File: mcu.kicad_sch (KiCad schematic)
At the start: 42 parts, among them SW1 TS-1088-AR02016, SW2 TS-1088-AR02016, SW3 TS-1088-AR02016, SW4 TS-1088-AR02016, U1 STM32H723VGTx, U14 AS5047P-ATST, U15 TCAN1044VDRQ1, U9 LSM6DSVTR, X1 X322512MSB4SI

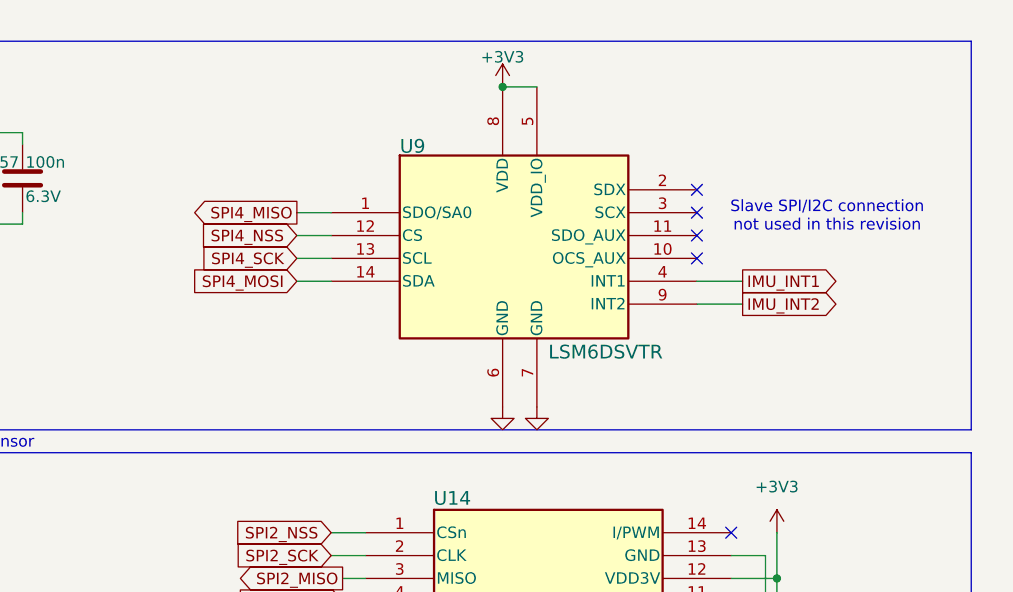
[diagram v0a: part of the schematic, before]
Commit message: wip gate driver change
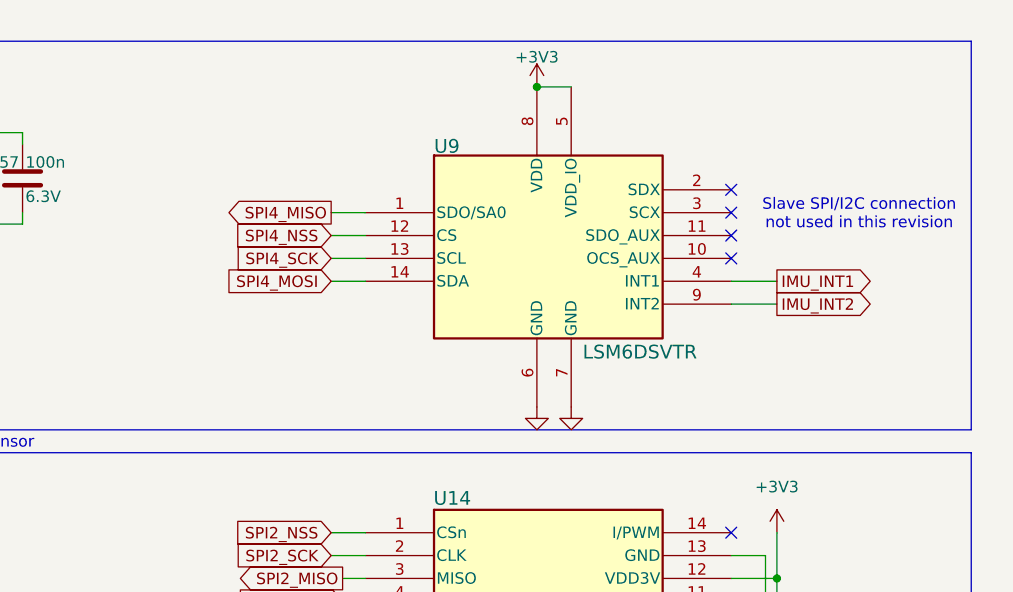
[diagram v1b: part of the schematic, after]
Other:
- moved on the sheet: U9
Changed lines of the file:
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@@
 	(text "Slave SPI/I2C connection\nnot used in this revision"
 		(exclude_from_sim no)
-		(at 265.938 34.798 0)
+		(at 269.494 34.544 0)
 		(effects
 			(font
@@
 	)
 	(junction
-		(at 229.87 20.32)
+		(at 233.68 20.32)
 		(diameter 0)
 		(color 0 0 0 0)
@@
 	)
 	(no_connect
-		(at 251.46 39.37)
+		(at 255.27 39.37)
 	)
 	(no_connect
-		(at 251.46 36.83)
+		(at 255.27 36.83)
 	)
 	(no_connect
@@
 	)
 	(no_connect
-		(at 251.46 31.75)
+		(at 255.27 31.75)
 	)
 	(no_connect
@@
 	)
 	(no_connect
-		(at 251.46 34.29)
+		(at 255.27 34.29)
 	)
 	(no_connect
@@
 	(wire
 		(pts
-			(xy 207.01 39.37) (xy 210.82 39.37)
+			(xy 210.82 39.37) (xy 214.63 39.37)
 		)
 		(stroke
@@
 	(wire
 		(pts
-			(xy 207.01 41.91) (xy 210.82 41.91)
+			(xy 210.82 41.91) (xy 214.63 41.91)
 		)
 		(stroke
@@
 	(wire
 		(pts
-			(xy 229.87 20.32) (xy 233.68 20.32)
+			(xy 233.68 20.32) (xy 237.49 20.32)
 		)
 		(stroke
@@
 	(wire
 		(pts
-			(xy 251.46 44.45) (xy 256.54 44.45)
+			(xy 255.27 44.45) (xy 260.35 44.45)
 		)
 		(stroke
@@
 	(wire
 		(pts
-			(xy 251.46 41.91) (xy 256.54 41.91)
+			(xy 255.27 41.91) (xy 260.35 41.91)
 		)
 		(stroke
@@
 	(wire
 		(pts
-			(xy 207.01 34.29) (xy 210.82 34.29)
+			(xy 210.82 34.29) (xy 214.63 34.29)
 		)
 		(stroke
@@
 	(wire
 		(pts
-			(xy 207.01 36.83) (xy 210.82 36.83)
+			(xy 210.82 36.83) (xy 214.63 36.83)
 		)
 		(stroke
@@
 	(global_label "SPI4_MOSI"
 		(shape input)
-		(at 207.01 41.91 180)
+		(at 210.82 41.91 180)
 		(fields_autoplaced yes)
 		(effects
@@
 		)
 		(property "Intersheetrefs" "${INTERSHEET_REFS}"
-			(at 194.1672 41.91 0)
+			(at 197.9772 41.91 0)
 			(effects
 				(font
@@
 	(global_label "IMU_INT2"
 		(shape output)
-		(at 256.54 44.45 0)
+		(at 260.35 44.45 0)
 		(fields_autoplaced yes)
 		(effects
@@
 		)
 		(property "Intersheetrefs" "${INTERSHEET_REFS}"
-			(at 267.9919 44.45 0)
+			(at 271.8019 44.45 0)
 			(effects
 				(font
@@
 	(global_label "SPI4_SCK"
 		(shape input)
-		(at 207.01 39.37 180)
+		(at 210.82 39.37 180)
 		(fields_autoplaced yes)
 		(effects
@@
 		)
 		(property "Intersheetrefs" "${INTERSHEET_REFS}"
-			(at 195.0139 39.37 0)
+			(at 198.8239 39.37 0)
 			(effects
 				(font
@@
 	(global_label "IMU_INT1"
 		(shape output)
-		(at 256.54 41.91 0)
+		(at 260.35 41.91 0)
 		(fields_autoplaced yes)
 		(effects
@@
 		)
 		(property "Intersheetrefs" "${INTERSHEET_REFS}"
-			(at 267.9919 41.91 0)
+			(at 271.8019 41.91 0)
 			(effects
 				(font
@@
 	(global_label "SPI4_MISO"
 		(shape output)
-		(at 207.01 34.29 180)
+		(at 210.82 34.29 180)
 		(fields_autoplaced yes)
 		(effects
@@
 		)
 		(property "Intersheetrefs" "${INTERSHEET_REFS}"
-			(at 194.1672 34.29 0)
+			(at 197.9772 34.29 0)
 			(effects
 				(font
@@
 	(global_label "SPI4_NSS"
 		(shape input)
-		(at 207.01 36.83 180)
+		(at 210.82 36.83 180)
 		(fields_autoplaced yes)
 		(effects
@@
 		)
 		(property "Intersheetrefs" "${INTERSHEET_REFS}"
-			(at 195.0139 36.83 0)
+			(at 198.8239 36.83 0)
 			(effects
 				(font
@@
 	(symbol
 		(lib_id "power:+3V3")
-		(at 229.87 20.32 0)
+		(at 233.68 20.32 0)
 		(unit 1)
 		(exclude_from_sim no)
@@
 		(dnp no)
 		(property "Reference" "#PWR0134"
-			(at 229.87 24.13 0)
+			(at 233.68 24.13 0)
 			(effects
 				(font
@@
 		)
 		(property "Value" "+3V3"
-			(at 229.87 17.018 0)
+			(at 233.68 17.018 0)
 			(effects
 				(font
@@
 		)
 		(property "Footprint" ""
-			(at 229.87 20.32 0)
+			(at 233.68 20.32 0)
 			(effects
 				(font
@@
 		)
 		(property "Datasheet" ""
-			(at 229.87 20.32 0)
+			(at 233.68 20.32 0)
 			(effects
 				(font
@@
 		)
 		(property "Description" "Power symbol creates a global label with name \"+3V3\""
-			(at 229.87 20.32 0)
+			(at 233.68 20.32 0)
 			(effects
 				(font
@@
 	(symbol
 		(lib_id "power:GND")
-		(at 229.87 55.88 0)
+		(at 233.68 55.88 0)
 		(unit 1)
 		(exclude_from_sim no)
@@
 		(fields_autoplaced yes)
 		(property "Reference" "#PWR082"
-			(at 229.87 62.23 0)
+			(at 233.68 62.23 0)
 			(effects
 				(font
@@
 		)
 		(property "Value" "GND"
-			(at 229.87 60.96 0)
+			(at 233.68 60.96 0)
 			(effects
 				(font
@@
 		)
 		(property "Footprint" ""
-			(at 229.87 55.88 0)
+			(at 233.68 55.88 0)
 			(effects
 				(font
@@
 		)
 		(property "Datasheet" ""
-			(at 229.87 55.88 0)
+			(at 233.68 55.88 0)
 			(effects
 				(font
@@
 		)
 		(property "Description" "Power symbol creates a global label with name \"GND\" , ground"
-			(at 229.87 55.88 0)
+			(at 233.68 55.88 0)
 			(effects
 				(font
@@
 	(symbol
 		(lib_id "NanoGaN:LSM6DSVTR")
-		(at 210.82 30.48 0)
+		(at 214.63 30.48 0)
 		(unit 1)
 		(exclude_from_sim no)
@@
 		(dnp no)
 		(property "Reference" "U9"
-			(at 218.44 26.924 0)
+			(at 222.25 26.924 0)
 			(effects
 				(font
@@
 		)
 		(property "Value" "LSM6DSVTR"
-			(at 234.95 49.784 0)
+			(at 238.76 49.784 0)
 			(effects
 				(font
@@
 		)
 		(property "Footprint" "NanoGaN:LGA14-L_2P59X3P1X0P5_STM-L"
-			(at 267.462 54.864 0)
+			(at 271.272 54.864 0)
 			(effects
 				(font
@@
 		)
 		(property "Datasheet" "LSM6DSVTR"
-			(at 258.572 56.896 0)
+			(at 262.382 56.896 0)
 			(effects
 				(font
@@
 		)
 		(property "Description" "-40℃~+85℃ 1.71V~3.6V 2.6uA 4.5KB IMU SPI、I2C、I3C X,Y,Z X,Y,Z ±16g ±4000dps LGA-14L(2.5x3) Accelerometers ROHS"
-			(at 307.086 59.436 0)
+			(at 310.896 59.436 0)
 			(effects
 				(font
@@
 		)
 		(property "LCSC" "C41785564"
-			(at 255.524 62.484 0)
+			(at 259.334 62.484 0)
 			(effects
 				(font
@@
 	(symbol
 		(lib_id "power:GND")
-		(at 233.68 55.88 0)
+		(at 237.49 55.88 0)
 		(unit 1)
 		(exclude_from_sim no)
@@
 		(fields_autoplaced yes)
 		(property "Reference" "#PWR0133"
-			(at 233.68 62.23 0)
+			(at 237.49 62.23 0)
 			(effects
 				(font
@@
 		)
 		(property "Value" "GND"
-			(at 233.68 60.96 0)
+			(at 237.49 60.96 0)
 			(effects
 				(font
@@
 		)
 		(property "Footprint" ""
-			(at 233.68 55.88 0)
+			(at 237.49 55.88 0)
 			(effects
 				(font
@@
 		)
 		(property "Datasheet" ""
-			(at 233.68 55.88 0)
+			(at 237.49 55.88 0)
 			(effects
 				(font
@@
 		)
 		(property "Description" "Power symbol creates a global label with name \"GND\" , ground"
-			(at 233.68 55.88 0)
+			(at 237.49 55.88 0)
 			(effects
 				(font
